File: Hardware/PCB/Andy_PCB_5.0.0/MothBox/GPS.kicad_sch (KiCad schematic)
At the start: 49 parts, among them U1 Days, U17 GPs 5 pin PM2.54-1*5, U2 Hours1, U6 Hours2, U7 Modes, U8 CD74HC4067M96E4, U9 CD74HC4067M96E4

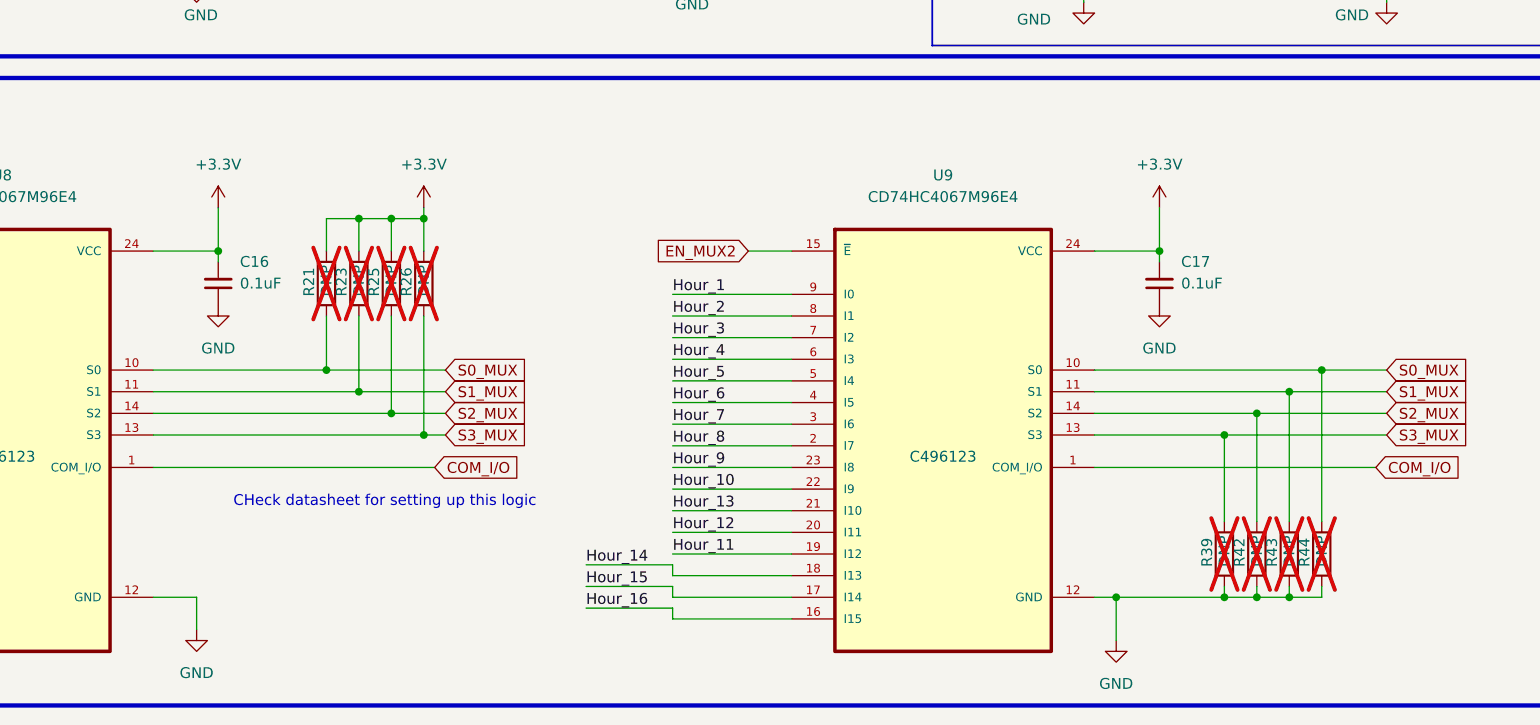
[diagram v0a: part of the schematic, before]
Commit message: before i kill the pullup resistors
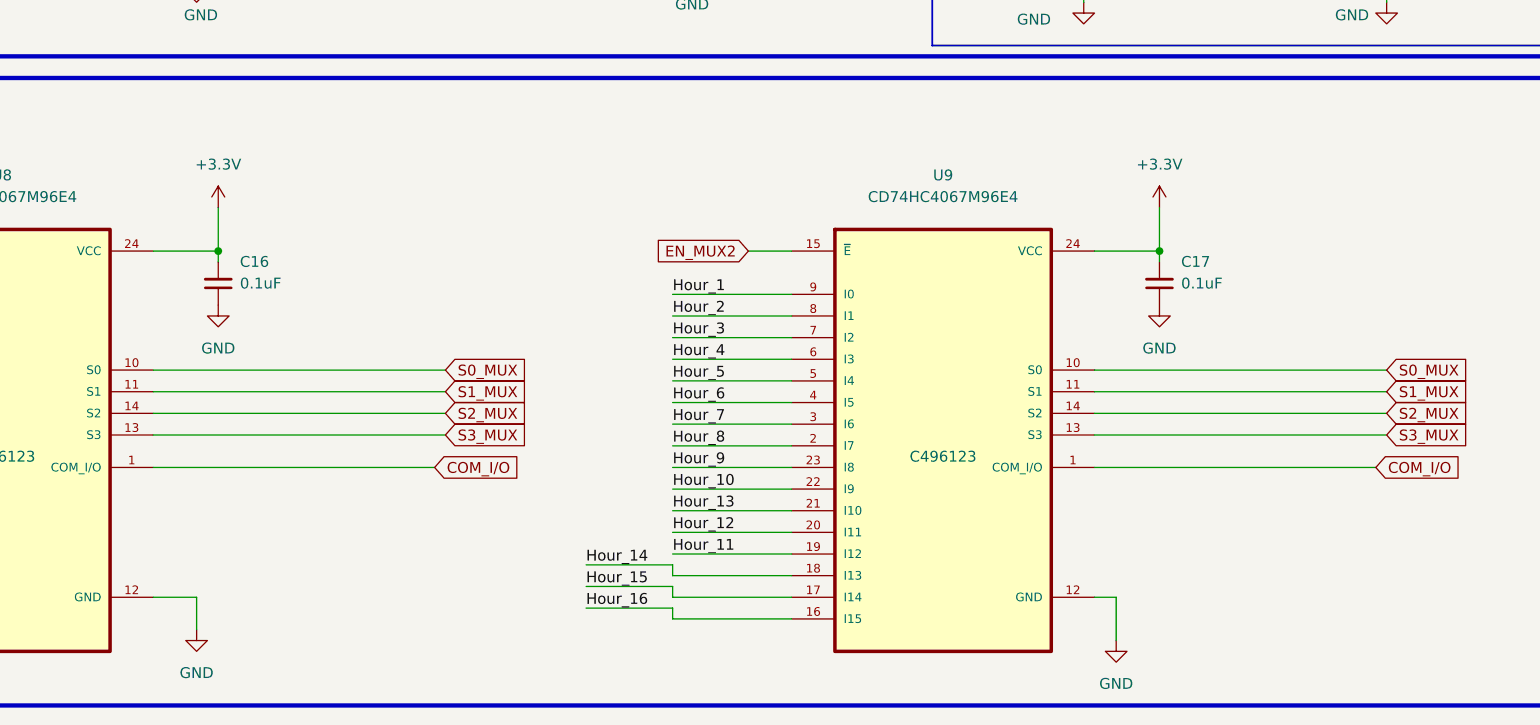
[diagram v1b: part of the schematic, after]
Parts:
- removed R21, R23, R25, R26, R39, R42, R43, R44: DNP, Resistor_SMD:R_0805_2012Metric, symbol Device:R
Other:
- note removed: "CHeck datasheet for setting up this logic"
